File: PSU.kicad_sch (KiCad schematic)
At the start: 56 parts, among them U11 TPSM84338, U13 TPS26400PWPR, U14 TPS7A39, U18 TLV1117-33

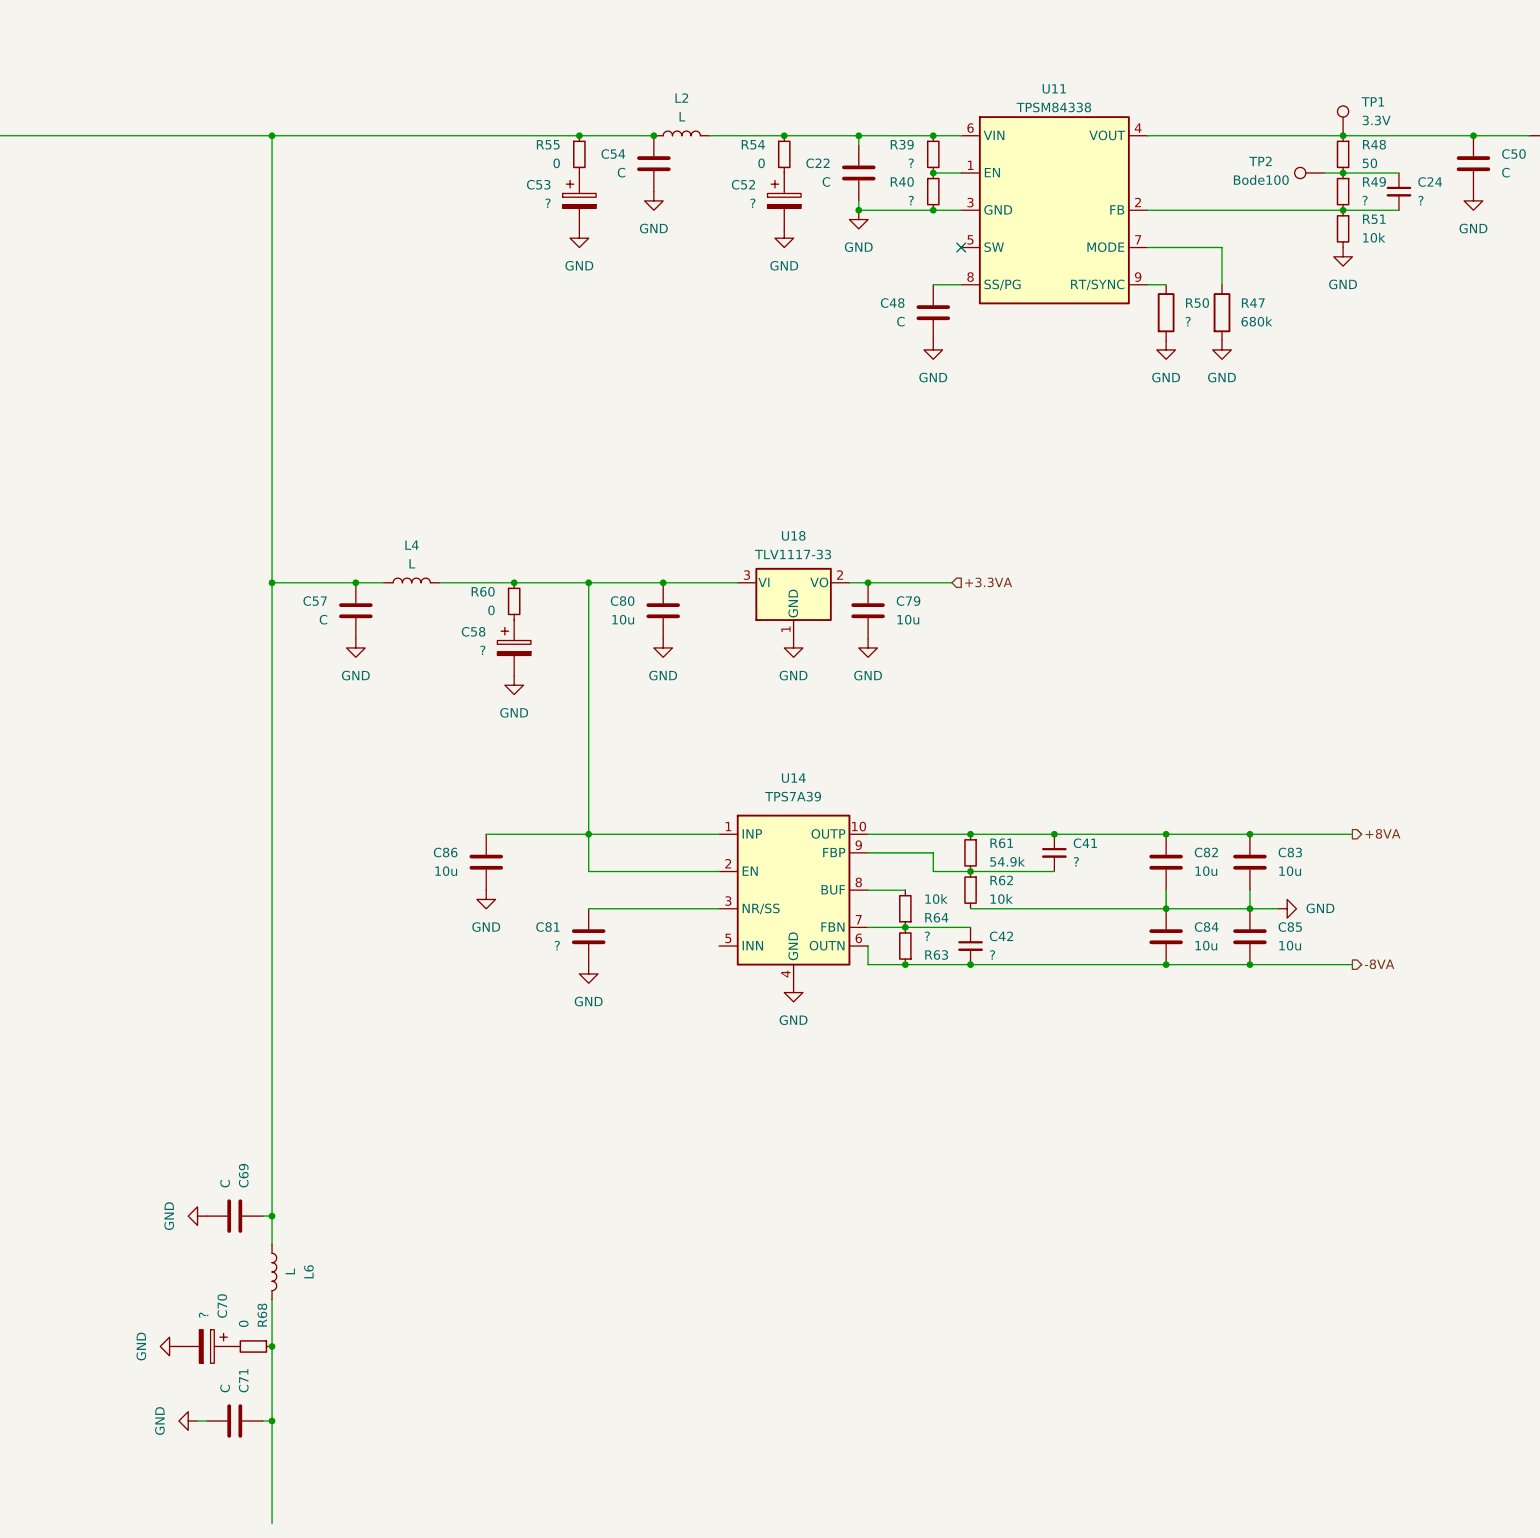
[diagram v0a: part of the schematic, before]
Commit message: modified:   MCU.kicad_sch 	modified:   PSU.kicad_sch 	modified:   ProjectY.kicad_pro 	modified:   ProjectY.kicad_sch 	modified:   ad.kicad_sch 	modified:   audio.kicad_sch
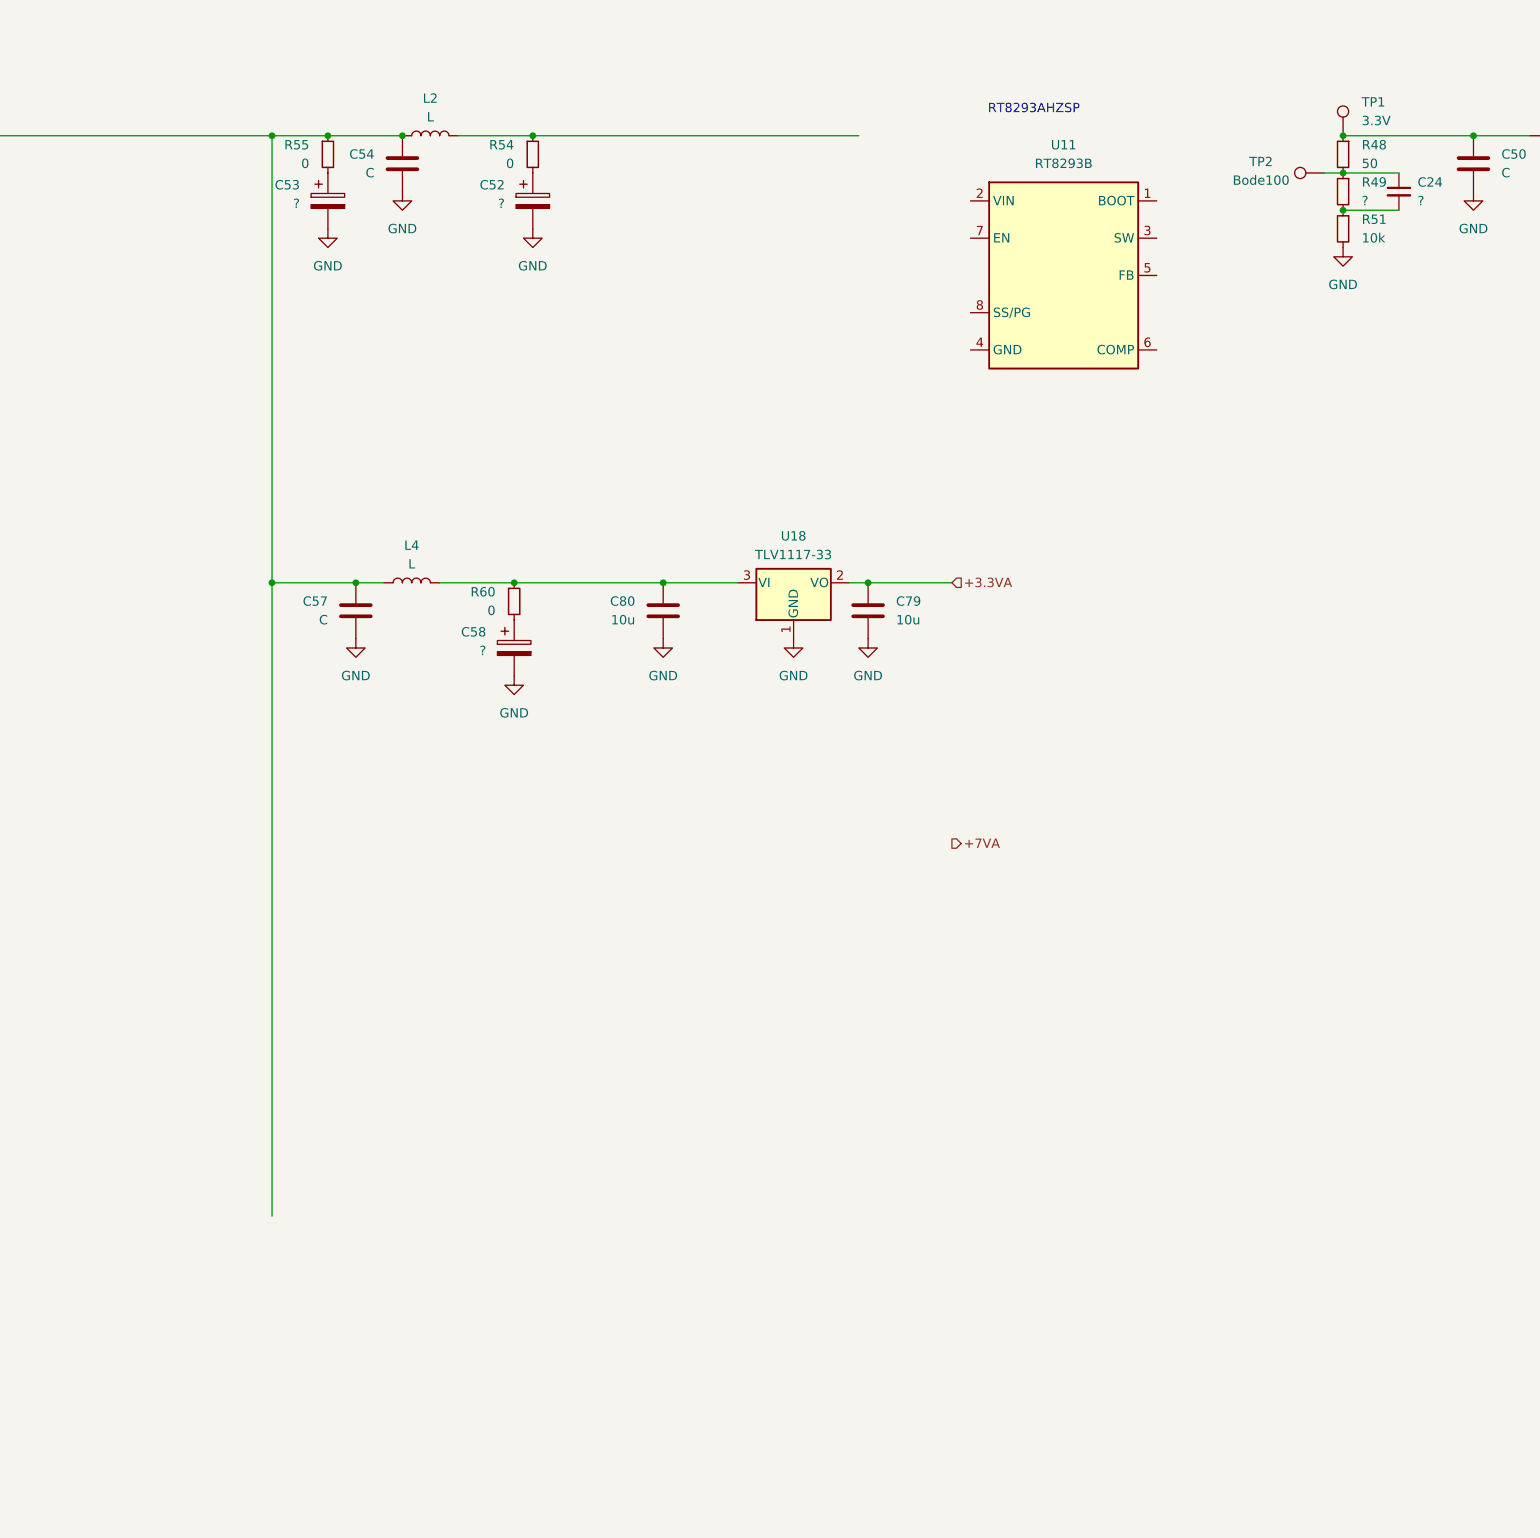
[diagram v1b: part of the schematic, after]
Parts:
- removed C22, C48, C69, C71: C, symbol Device:C
- removed C41, C42: ?, symbol Device:C_Small
- removed C70: ?, symbol Device:C_Polarized
- removed C81: ?, symbol Device:C
- removed C82, C83, C84, C85, C86: 10u, symbol Device:C
- removed L6: L, symbol Device:L
- removed R39, R40, R63: ?, symbol Device:R_Small
- removed R47: 680k, symbol Device:R
- removed R50: ?, symbol Device:R
- removed R61: 54.9k, symbol Device:R_Small
- removed R62, R64: 10k, symbol Device:R_Small
- removed R68: 0, symbol Device:R_Small
- removed U11: TPSM84338, symbol User:TPSM84338_
- removed U14: TPS7A39, Package_SON:Texas_S-PVSON-N10_ThermalVias, symbol Regulator_Linear:TPS7A39
- added U11: RT8293B, symbol User:RT8293B
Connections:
- net GND: now also U11.4 (GND), U11.9 (GND)
- no-connect marks 5 -> 4
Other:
- note added: "RT8293AHZSP"
- moved on the sheet: C52, C53, C54, L2, R54, R55

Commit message: modified:   MCU.kicad_sch 	modified:   PSU.kicad_sch 	modified:   ProjectY.kicad_pro 	modified:   ProjectY.kicad_sch 	modified:   audio.kicad_sch 	modified:   fp-info-cache 	new file:   spdif.kicad_sch 	modified:   usbfilter.kicad_sch
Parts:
- removed C53, C58: ?, symbol Device:C_Polarized
- removed C56: Css, symbol Device:C_Polarized_Small
- removed C57: C, symbol Device:C
- removed C79, C80: 10u, symbol Device:C
- removed D1: D_TVS, symbol Device:D_TVS
- removed L3: Choke_Wurth_WE-CNSW_744232090, Inductor_SMD:L_CommonMode_Wurth_WE-CNSW-1206, symbol Filter:Choke_Wurth_WE-CNSW_744232090
- removed L4: L, symbol Device:L
- removed R54, R55, R60: 0, symbol Device:R_Small
- removed R57, R58, R59: ?, symbol Device:R_Small
- removed U13: TPS26400PWPR, PWP0016H-IPC_A, symbol 2025-02-23_17-32-12:TPS26400PWPR
- removed U18: TLV1117-33, symbol Regulator_Linear:TLV1117-33
- added C3, C4, C5, C6, C7, C9: 10uF, PCM_JLCPCB:C_0603, symbol PCM_JLCPCB-Capacitors:0603,10uF,(2)
- added C49: C, symbol Device:C
- added D1: 1N4148W, PCM_JLCPCB:D_SOD-123, symbol PCM_JLCPCB-Diodes:Switching,1N4148W
- added FB1, FB2: FerriteBead, symbol Device:FerriteBead
- added L1: Choke_Wurth_WE-CNSW_744232090, Inductor_SMD:L_CommonMode_Wurth_WE-CNSW-1206, symbol Filter:Choke_Wurth_WE-CNSW_744232090
- added R10, R11: 5.1kΩ, PCM_JLCPCB:R_0402, symbol PCM_JLCPCB-Resistors:0402,5.1kΩ
- added R12: 0Ω, PCM_JLCPCB:R_0402, symbol PCM_JLCPCB-Resistors:0402,0Ω
- added U12: USBLC6-2P6, Package_TO_SOT_SMD:SOT-666, symbol Power_Protection:USBLC6-2P6
- added U4: TPS7A39, Package_SON:Texas_S-PVSON-N10_ThermalVias, symbol Regulator_Linear:TPS7A39
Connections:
- net +3.3V: now also C50.1, FB3.1, R48.1, TP1.1, U11.5 (FB); no longer C51.1, FB3.2, R56.1
- net +9V: now also C3.1, C4.1, C5.1, C6.1, C7.1, C9.1
- net GND: now also C3.2, C4.2, C49.2, C5.2, C6.2, C7.2, C9.2, R10.1, R11.1, U12.2 (GND)
- net at U11.2 (VIN): now also L2.2
- net at C52.1: now also R12.2
- net +9V_protected: no longer names the net of C54.1, L2.1
- new net: C51.1, FB3.2, R56.1
- new net: L1.2, U12.1 (I/O1)
- new net: L1.3, U12.3 (I/O2)
- new net: D1.2, FB2.2
- new net: U4.11 (GND), U4.4 (GND)
- new net: C49.1, FB1.2, FB2.1
- new net CC: R10.2
- new net D+: U12.6 (I/O1)
- new net D-: U12.4 (I/O2)
- new net Dfiltered+: L1.1
- new net Dfiltered-: L1.4
- new net VBUS: FB1.1, U12.5 (VBUS)
- new net VBUS_detect: D1.1
- new net VCONN: R11.2
- no-connect marks 4 -> 0
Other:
- note added: "4-18V"
- note added: "OR controller"
- note added: "TPS65133"
- note removed: "RT8293AHZSP"
- moved on the sheet: C24, C50, C51, C52, C54, C55, FB3, L2, R48, R49, R51, R56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

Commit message: asd
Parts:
- removed C24: ?, symbol Device:C_Small
- removed C3, C4, C5, C6, C7: 10uF, PCM_JLCPCB:C_0603, symbol PCM_JLCPCB-Capacitors:0603,10uF,(2)
- removed C49: C, symbol Device:C
- removed D1: 1N4148W, PCM_JLCPCB:D_SOD-123, symbol PCM_JLCPCB-Diodes:Switching,1N4148W
- removed FB1, FB2: FerriteBead, symbol Device:FerriteBead
- removed R48: 50, symbol Device:R_Small
- removed R49: ?, symbol Device:R_Small
- removed R51: 10k, symbol Device:R_Small
- removed TP1: 3.3V, symbol Connector:TestPoint
- removed TP2: Bode100, symbol Connector:TestPoint
- added C14, C64: 10uF, PCM_JLCPCB:C_0603, symbol PCM_JLCPCB-Capacitors:0603,10uF,(2)
- added C24: DNP, Capacitor_SMD:C_0805_2012Metric, symbol Device:C
- added C25, C58, C59, C60, C61, C62, C68, C69: 10uF, PCM_JLCPCB:C_0402, symbol PCM_JLCPCB-Capacitors:0402,10uF
- added C26, C33, C41, C42, C48, C49, C5, C6, C7: 10uF, PCM_JLCPCB:C_0603, symbol PCM_JLCPCB-Capacitors:0603,10uF
- added C3, C4, C57: 100nF, PCM_JLCPCB:C_0402, symbol PCM_JLCPCB-Capacitors:0402,100nF,(2)
- added C53, C56: 100uF, PCM_JLCPCB:C_CASE-B-3528-21(mm), symbol PCM_JLCPCB-Capacitors:CASE-B-3528-21(mm),100uF
- added C63: 2.2nF, PCM_JLCPCB:C_0805, symbol PCM_JLCPCB-Capacitors:0805,2.2nF
- added C65, C66, C67: C, symbol Device:C
- added D1: SMF20CA, PCM_JLCPCB:D_SOD-123FL, symbol PCM_JLCPCB-Diodes:TVS-Uni,SMF20CA
- added L3: 3.6uH, symbol Device:L
- added L4, L5: XFL4020-472MEC, Inductor_SMD:L_Coilcraft_XxL4020, symbol Device:L
- added Q1: DMT6008LFG, Package_SON:Diodes_PowerDI3333-8, symbol Transistor_FET:DMT6008LFG
- added R36: 4.7kΩ, PCM_JLCPCB:R_0402, symbol PCM_JLCPCB-Resistors:0402,4.7kΩ
- added R39, R57, R58, R60: 10kΩ, PCM_JLCPCB:R_0402, symbol PCM_JLCPCB-Resistors:0402,10kΩ
- added R46: 22kΩ, PCM_JLCPCB:R_0402, symbol PCM_JLCPCB-Resistors:0402,22kΩ
- added R47: 47kΩ, PCM_JLCPCB:R_0402, symbol PCM_JLCPCB-Resistors:0402,47kΩ
- added R48, R51, R53, R55: 4.7kΩ, PCM_JLCPCB:R_0603, symbol PCM_JLCPCB-Resistors:0603,4.7kΩ
- added R49, R50, R52, R54, R59, R61: R, symbol Device:R
- added U17: TPS2121RUXR, User:IC_TPS2121RUXR, symbol User:TPS2121RUXR
- added U19: TLV77333PDBVR, Package_TO_SOT_SMD:SOT-23-5, symbol Regulator_Linear:AP2127K-3.3
- added U20: TPS65133DPDR, User:SON40P300X300X80-13N, symbol User:TPS65133DPDR
- added U21: LM74700, Package_TO_SOT_SMD:SOT-23-6, symbol Power_Management:LM74700
- added U22: TLV77325PDBVR, Package_TO_SOT_SMD:SOT-23-5, symbol Regulator_Linear:AP2127K-3.3
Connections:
- net GND is gone; now on net AGND: C50.2, C51.2, C52.2, C54.2, C55.2, C9.2, R10.1, R11.1, U11.4 (GND), U11.9 (GND), U12.2 (GND)
- net +3.3V: now also C58.1, C59.1, C60.1, C61.1, C62.1, C68.1, L3.2, R57.1, U22.1 (VIN), U22.3 (EN); no longer U11.5 (FB)
- net +9V: now also C3.1, C4.1, D1.1, Q1.1 (S), Q1.2 (S), Q1.3 (S), U21.3 (EN), U21.6 (ANODE); no longer C9.1
- net VBUS: now also C14.2, R36.1, R52.1, R54.1, U17.2 (IN2), U17.2_1 (IN2__1)
- net VIN_FILT: now reaches R12.1
- net VIN_FILT: now also L2.2, U11.2 (VIN), C65.1
- net AVIN: now reaches C51.1, FB3.2, R56.1
- net AVIN: now also L5.2, U20.11 (AVIN), U20.12 (PVIN), U20.7 (EN)
- net at U11.1 (BOOT): now also C57.1
- net at U11.3 (SW): now also C57.2, L3.1
- net at U11.6 (COMP): now also C24.1, R46.1
- net VIN_4V-18V: now reaches C54.1, L2.1
- net VIN_4V-18V: now also U17.1 (OUT), U17.1_1 (OUT__1), U17.8 (OUT__2), U17.8_1 (OUT__3)
- net +5V: now reaches U4.1 (INP)
- net +5V: now also U4.2 (EN), C26.1, C41.1, C48.1, C5.1, C6.1, U19.1 (VIN), U19.3 (EN), U20.3 (VPOS)
- net +4.5V: now reaches U4.10 (OUTP)
- net +4.5V: now also C53.1, C66.1, R59.1
- net AGND: now reaches U4.11 (GND), U4.4 (GND)
- net AGND: now also C14.1, C24.2, C25.2, C26.2, C3.2, C33.1, C41.2, C42.1, C48.2, C49.1, C5.2, C53.2, C56.1, C58.2, C59.2, C6.2, C60.2, C61.2, C62.2, C63.2, C64.2, C65.2, C68.2, C69.2, C7.1, D1.2, L4.1, R39.2, R47.2, R48.2, R51.2, R53.2, R55.2, R58.2, U17.12 (GND), U19.2 (GND), U19.4 (NC), U20.13 (EP), U20.2 (PGND), U20.4 (GND), U20.5 (AGND), U20.6 (GND__1), U20.8 (GND__2), U21.2 (GND), U22.2 (GND), U22.4 (NC)
- net -5V: now reaches U4.5 (INN)
- net -5V: now also C33.2, C42.2, C49.2, C7.2, U20.9 (VNEG)
- net -4.5V: now reaches U4.6 (OUTN)
- net -4.5V: now also C56.2, C67.2, R61.2
- net FBN: now reaches U4.7 (FBN)
- net FBN: now also C67.1, R60.2, R61.1
- net BUF: now reaches U4.8 (BUF)
- net BUF: now also R60.1
- net FBP: now reaches U4.9 (FBP)
- net FBP: now also C66.2, R58.1, R59.2
- new net: R52.2, R53.1, U17.4 (OV2)
- new net: L4.2, U20.10 (SWN)
- new net: C4.2, U21.1 (VCAP)
- new net: Q1.4 (G), U21.5 (GATE)
- new net: R50.2, R51.1, U17.5 (OV1)
- new net: C63.1, R46.2
- new net: L5.1, U20.1 (SWP)
- new net: R47.1, U17.10 (ILIM)
- new net: C64.1, U17.11 (SS)
- new net +2.5VA: C69.1, U22.5 (VOUT)
- new net +3.3VA: C25.1, U19.5 (VOUT)
- new net +9V_REVERSE_PROTECTED: C9.1, Q1.5 (D), R49.1, R50.1, U17.7 (IN1), U17.7_1 (IN1__1), U21.4 (CATHODE)
- new net CP2: R54.2, R55.1, U17.3 (CP2)
- new net PR1: R48.1, R49.2, U17.6 (PR1)
- new net PSU_ST: R57.2, U17.9 (ST)
- new net VBUS_DETECT: R36.2, R39.1
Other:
- note removed: "4-18V"
- note removed: "OR controller"
- note removed: "TPS65133"
- moved on the sheet: C50, C51, C52, C54, C55, C9, FB3, L2, R12, R56, U11, U4
